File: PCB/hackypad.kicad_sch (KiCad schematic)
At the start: 21 parts, among them SW1 SW_Push_45deg, SW10 RotaryEncoder_Switch, SW2 SW_Push_45deg, SW3 SW_Push_45deg, SW4 SW_Push_45deg, SW5 SW_Push_45deg, SW6 SW_Push_45deg, SW7 SW_Push_45deg, SW8 SW_Push_45deg, SW9 SW_Push_45deg, U1 MOUDLE-SEEEDUINO-XIAO, U2 ER_OLEDM0.91_1x-I2C

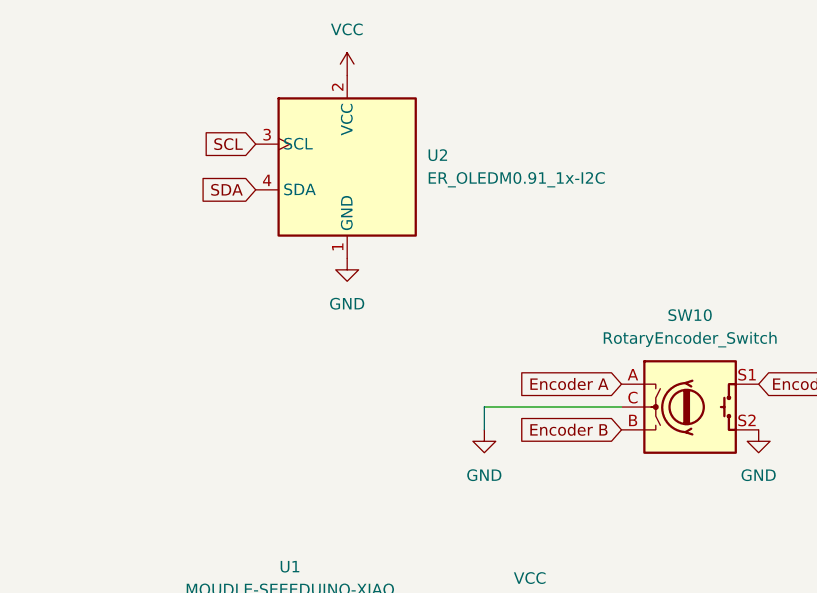
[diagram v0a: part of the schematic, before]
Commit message: feat(PCB): Add 3d models
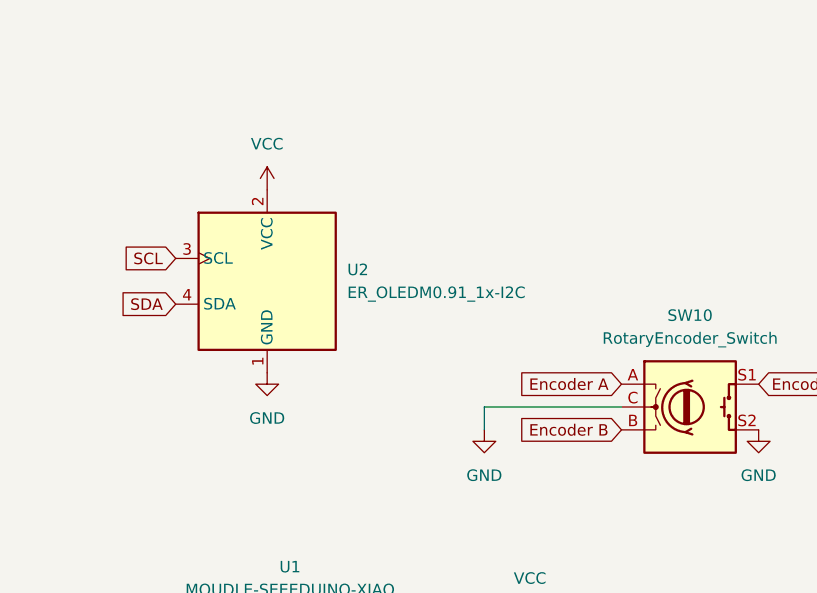
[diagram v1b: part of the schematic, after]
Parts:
- SW1, SW2, SW3, SW4, SW5, SW6, SW7, SW8, SW9: footprint Button_Switch_Keyboard:SW_Cherry_MX_1.00u_PCB -> switch:SW_Cherry_MX_1.00u_PCB
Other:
- moved on the sheet: U2
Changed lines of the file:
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@@
 	(global_label "SDA"
 		(shape input)
-		(at 50.8 29.21 180)
+		(at 41.91 41.91 180)
 		(fields_autoplaced yes)
 		(effects
@@
 		)
 		(property "Intersheetrefs" "${INTERSHEET_REFS}"
-			(at 44.2467 29.21 0)
+			(at 35.3567 41.91 0)
 			(hide yes)
 			(show_name no)
@@
 	(global_label "SCL"
 		(shape input)
-		(at 50.8 24.13 180)
+		(at 41.91 36.83 180)
 		(fields_autoplaced yes)
 		(effects
@@
 		)
 		(property "Intersheetrefs" "${INTERSHEET_REFS}"
-			(at 44.3072 24.13 0)
+			(at 35.4172 36.83 0)
 			(hide yes)
 			(show_name no)
@@
 	(symbol
 		(lib_id "power:VCC")
-		(at 60.96 16.51 0)
+		(at 52.07 29.21 0)
 		(unit 1)
 		(body_style 1)
@@
 		(fields_autoplaced yes)
 		(property "Reference" "#PWR05"
-			(at 60.96 20.32 0)
+			(at 52.07 33.02 0)
 			(hide yes)
 			(show_name no)
@@
 		)
 		(property "Value" "VCC"
-			(at 60.96 11.43 0)
+			(at 52.07 24.13 0)
 			(show_name no)
 			(do_not_autoplace no)
@@
 		)
 		(property "Footprint" ""
-			(at 60.96 16.51 0)
+			(at 52.07 29.21 0)
 			(hide yes)
 			(show_name no)
@@
 		)
 		(property "Datasheet" ""
-			(at 60.96 16.51 0)
+			(at 52.07 29.21 0)
 			(hide yes)
 			(show_name no)
@@
 		)
 		(property "Description" "Power symbol creates a global label with name \"VCC\""
-			(at 60.96 16.51 0)
+			(at 52.07 29.21 0)
 			(hide yes)
 			(show_name no)
@@
 			)
 		)
-		(property "Footprint" "Button_Switch_Keyboard:SW_Cherry_MX_1.00u_PCB"
+		(property "Footprint" "switch:SW_Cherry_MX_1.00u_PCB"
 			(at 137.16 106.68 0)
 			(hide yes)
@@
 	(symbol
 		(lib_id "power:GND")
-		(at 60.96 36.83 0)
+		(at 52.07 49.53 0)
 		(unit 1)
 		(body_style 1)
@@
 		(fields_autoplaced yes)
 		(property "Reference" "#PWR04"
-			(at 60.96 43.18 0)
+			(at 52.07 55.88 0)
 			(hide yes)
 			(show_name no)
@@
 		)
 		(property "Value" "GND"
-			(at 60.96 41.91 0)
+			(at 52.07 54.61 0)
 			(show_name no)
 			(do_not_autoplace no)
@@
 		)
 		(property "Footprint" ""
-			(at 60.96 36.83 0)
+			(at 52.07 49.53 0)
 			(hide yes)
 			(show_name no)
@@
 		)
 		(property "Datasheet" ""
-			(at 60.96 36.83 0)
+			(at 52.07 49.53 0)
 			(hide yes)
 			(show_name no)
@@
 		)
 		(property "Description" "Power symbol creates a global label with name \"GND\" , ground"
-			(at 60.96 36.83 0)
+			(at 52.07 49.53 0)
 			(hide yes)
 			(show_name no)
@@
 	(symbol
 		(lib_id "Display_Graphic:ER_OLEDM0.91_1x-I2C")
-		(at 60.96 26.67 0)
+		(at 52.07 39.37 0)
 		(unit 1)
 		(body_style 1)
@@
 		(fields_autoplaced yes)
 		(property "Reference" "U2"
-			(at 69.85 25.3999 0)
+			(at 60.96 38.0999 0)
 			(show_name no)
 			(do_not_autoplace no)
@@
 		)
 		(property "Value" "ER_OLEDM0.91_1x-I2C"
-			(at 69.85 27.9399 0)
+			(at 60.96 40.6399 0)
 			(show_name no)
 			(do_not_autoplace no)
@@
 		)
 		(property "Footprint" "Display:ER_OLEDM0.91_1x-I2C"
-			(at 78.994 39.37 0)
+			(at 70.104 52.07 0)
 			(hide yes)
 			(show_name no)
@@
 		)
 		(property "Datasheet" "https://www.buydisplay.com/download/manual/ER-OLEDM0.91-1_Datasheet.pdf"
-			(at 103.632 41.402 0)
+			(at 94.742 54.102 0)
 			(hide yes)
 			(show_name no)
@@
 		)
 		(property "Description" "SSD1306 OLED module, 0.91 inch, 128x32, I2C"
-			(at 87.63 43.434 0)
+			(at 78.74 56.134 0)
 			(hide yes)
 			(show_name no)
@@
 			)
 		)
-		(property "Footprint" "Button_Switch_Keyboard:SW_Cherry_MX_1.00u_PCB"
+		(property "Footprint" "switch:SW_Cherry_MX_1.00u_PCB"
 			(at 153.67 83.82 0)
 			(hide yes)
@@
 			)
 		)
-		(property "Footprint" "Button_Switch_Keyboard:SW_Cherry_MX_1.00u_PCB"
+		(property "Footprint" "switch:SW_Cherry_MX_1.00u_PCB"
 			(at 170.18 106.68 0)
 			(hide yes)
@@
 			)
 		)
-		(property "Footprint" "Button_Switch_Keyboard:SW_Cherry_MX_1.00u_PCB"
+		(property "Footprint" "switch:SW_Cherry_MX_1.00u_PCB"
 			(at 137.16 83.82 0)
 			(hide yes)
@@
 			)
 		)
-		(property "Footprint" "Button_Switch_Keyboard:SW_Cherry_MX_1.00u_PCB"
+		(property "Footprint" "switch:SW_Cherry_MX_1.00u_PCB"
 			(at 170.18 129.54 0)
 			(hide yes)
@@
 			)
 		)
-		(property "Footprint" "Button_Switch_Keyboard:SW_Cherry_MX_1.00u_PCB"
+		(property "Footprint" "switch:SW_Cherry_MX_1.00u_PCB"
 			(at 170.18 83.82 0)
 			(hide yes)
@@
 			)
 		)
-		(property "Footprint" "Button_Switch_Keyboard:SW_Cherry_MX_1.00u_PCB"
+		(property "Footprint" "switch:SW_Cherry_MX_1.00u_PCB"
 			(at 153.67 129.54 0)
 			(hide yes)
@@
 			)
 		)
-		(property "Footprint" "Button_Switch_Keyboard:SW_Cherry_MX_1.00u_PCB"
+		(property "Footprint" "switch:SW_Cherry_MX_1.00u_PCB"
 			(at 153.67 106.68 0)
 			(hide yes)
@@
 			)
 		)
-		(property "Footprint" "Button_Switch_Keyboard:SW_Cherry_MX_1.00u_PCB"
+		(property "Footprint" "switch:SW_Cherry_MX_1.00u_PCB"
 			(at 137.16 129.54 0)
 			(hide yes)
